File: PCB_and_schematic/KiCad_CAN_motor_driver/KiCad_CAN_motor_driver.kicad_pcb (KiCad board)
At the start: 2 copper layers, 90.4 x 45.2 mm, 75 parts, among them J1 SWDIO, J2 UART, J3 POWER IN 24V, J4 MOTOR OUT, J5 CAN, J6 PWM_IN, Q1 BTN8982TA, Q2 BTN8982TA, U1 SN65HVD232, U2 LMR50410, U3 STM32F103C8Tx

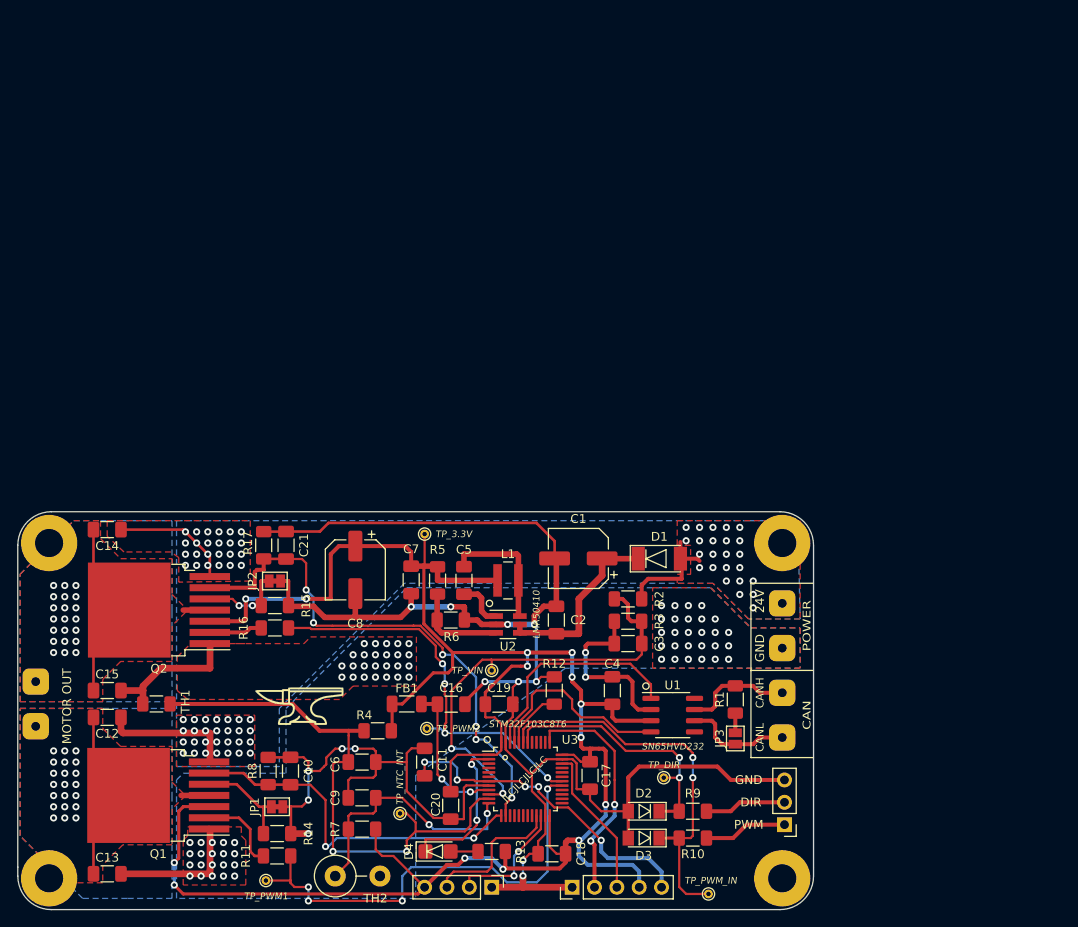
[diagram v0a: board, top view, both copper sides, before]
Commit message: PCB and schematic rev 1.1
+ revision 1.1 of schematic and PCB
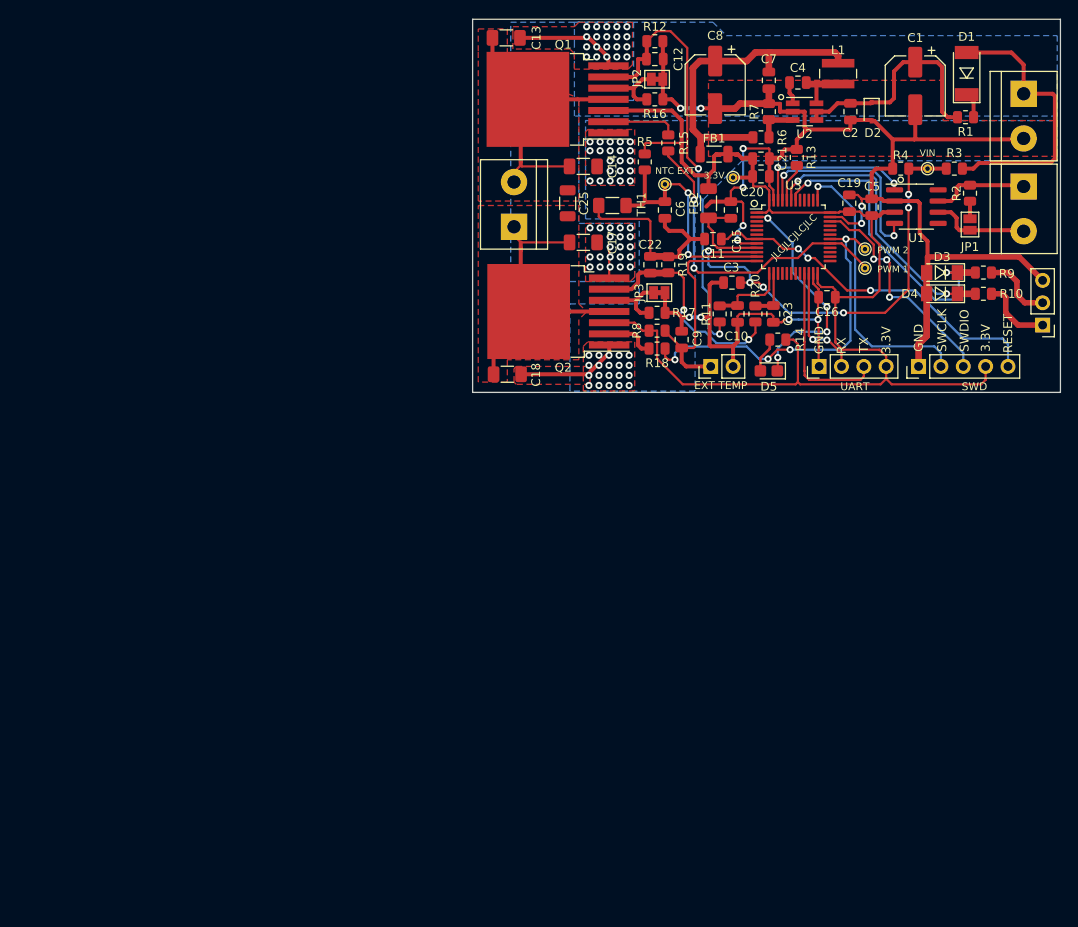
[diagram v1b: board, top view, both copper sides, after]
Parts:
- removed the G*** at (169.9, 81.0)
- removed the G*** at (137.9, 99.1)
- removed MountHole (x4): MountingHole_3.2mm_M3_Pad, MountingHole:MountingHole_3.2mm_M3_Pad
- removed REF**: OSHW-Logo2_7.3x6mm_SilkScreen, Symbol:OSHW-Logo2_7.3x6mm_SilkScreen
- removed REF**: KiCad-Logo2_5mm_SilkScreen, Symbol:KiCad-Logo2_5mm_SilkScreen
- removed TP_3.3V: 3V3, TestPoint:TestPoint_THTPad_D1.0mm_Drill0.5mm
- removed TP_DIR: DIR, TestPoint:TestPoint_THTPad_D1.0mm_Drill0.5mm
- removed TP_NTC_INT: NTC INT, TestPoint:TestPoint_THTPad_D1.0mm_Drill0.5mm
- removed TP_PWM1: PWM OUT 1, TestPoint:TestPoint_THTPad_D1.0mm_Drill0.5mm
- removed TP_PWM2: PWM OUT 2, TestPoint:TestPoint_THTPad_D1.0mm_Drill0.5mm
- removed TP_PWM_IN: PWM IN, TestPoint:TestPoint_THTPad_D1.0mm_Drill0.5mm
- removed TP_VIN: VIN, TestPoint:TestPoint_THTPad_D1.0mm_Drill0.5mm
- added C22: 10nF, Capacitor_SMD:C_0805_2012Metric, F.Cu at (177.8, 48.9)
- added C23: 10nF, Capacitor_SMD:C_0805_2012Metric, F.Cu at (191.8, 54.5)
- added C25: 100nF, Capacitor_SMD:C_1206_3216Metric, F.Cu at (168.4, 41.9)
- added D5: LED, LED_SMD:LED_0805_2012Metric_Castellated, F.Cu at (191.3, 61.0)
- added FB2: Ferrite_Bead, Inductor_SMD:L_1206_3216Metric_Pad1.22x1.90mm_HandSolder, F.Cu at (184.4, 41.9)
- added G***: LOGO, WK_lib:Anvil_10x10mm, B.Cu at (193.4, 24.1)
- added R18: 1k, Resistor_SMD:R_0805_2012Metric, F.Cu at (178.6, 58.4)
- added R19: 470R, Resistor_SMD:R_0805_2012Metric, F.Cu at (179.8, 48.9)
- added R20: 33k, Resistor_SMD:R_0805_2012Metric, F.Cu at (189.7, 54.5)
- added TP1: VIN, TestPoint:TestPoint_THTPad_D1.0mm_Drill0.5mm, F.Cu at (209.3, 38.0)
- added TP2: NTC INT, TestPoint:TestPoint_THTPad_D1.0mm_Drill0.5mm, F.Cu at (179.5, 39.8)
- added TP3: 3V3, TestPoint:TestPoint_THTPad_D1.0mm_Drill0.5mm, F.Cu at (187.2, 39.0)
- added TP5: PWM OUT 1, TestPoint:TestPoint_THTPad_D1.0mm_Drill0.5mm, F.Cu at (202.2, 49.3)
- added TP7: PWM OUT 2, TestPoint:TestPoint_THTPad_D1.0mm_Drill0.5mm, F.Cu at (202.2, 47.1)
- C10, C11, C16, C19, C2, C20, C3, C4, C5, C6, C7, C9: footprint Capacitor_SMD:C_1206_3216Metric_Pad1.33x1.80mm_HandSolder -> Capacitor_SMD:C_0805_2012Metric
- C12: value 220nF -> 10nF; footprint Capacitor_SMD:C_1206_3216Metric_Pad1.33x1.80mm_HandSolder -> Capacitor_SMD:C_0805_2012Metric
- C15: value 220nF -> 100nF; footprint Capacitor_SMD:C_1206_3216Metric_Pad1.33x1.80mm_HandSolder -> Capacitor_SMD:C_0805_2012Metric
- C17, C18: value 100nF -> 220nF
- C21: value 10nF -> 100nF; footprint Capacitor_SMD:C_1206_3216Metric_Pad1.33x1.80mm_HandSolder -> Capacitor_SMD:C_0805_2012Metric
- D2: value 3V -> SD24_SOD323; footprint Diode_SMD:D_MiniMELF -> Diode_SMD:D_SOD-323
- D4: value LED -> 3V; footprint LED_SMD:LED_1206_3216Metric_Castellated -> Diode_SMD:D_MiniMELF
- FB1: footprint Inductor_SMD:L_1206_3216Metric_Pad1.22x1.90mm_HandSolder -> Inductor_SMD:L_1206_3216Metric
- J3: value POWER IN 24V -> PWM_IN; footprint WK_lib:PowerPad_2x_3mm -> Connector_PinHeader_2.54mm:PinHeader_1x03_P2.54mm_Vertical
- J4: value MOTOR OUT -> POWER IN 24V; footprint WK_lib:PowerPad_2x_3mm -> WK_lib:ScrewTerminal_2_P5.08mm
- J5: value CAN -> MOTOR OUT; footprint WK_lib:PowerPad_2x_3mm -> WK_lib:ScrewTerminal_2_P5.08mm
- J6: value PWM_IN -> CAN; footprint Connector_PinHeader_2.54mm:PinHeader_1x03_P2.54mm_Vertical -> WK_lib:ScrewTerminal_2_P5.08mm
- JP1: footprint Jumper:SolderJumper-2_P1.3mm_Bridged_Pad1.0x1.5mm -> Jumper:SolderJumper-2_P1.3mm_Open_Pad1.0x1.5mm
- JP3: footprint Jumper:SolderJumper-2_P1.3mm_Open_Pad1.0x1.5mm -> Jumper:SolderJumper-2_P1.3mm_Bridged_Pad1.0x1.5mm
- R1: value 120R -> 10R; footprint Resistor_SMD:R_1206_3216Metric_Pad1.30x1.75mm_HandSolder -> Resistor_SMD:R_0805_2012Metric
- R10, R17, R9: footprint Resistor_SMD:R_1206_3216Metric_Pad1.30x1.75mm_HandSolder -> Resistor_SMD:R_0805_2012Metric
- R11: value 1k -> 33k; footprint Resistor_SMD:R_1206_3216Metric_Pad1.30x1.75mm_HandSolder -> Resistor_SMD:R_0805_2012Metric
- R12: value 10k -> 470R; footprint Resistor_SMD:R_1206_3216Metric_Pad1.30x1.75mm_HandSolder -> Resistor_SMD:R_0805_2012Metric
- R13: value 1.5k -> 10k; footprint Resistor_SMD:R_1206_3216Metric_Pad1.30x1.75mm_HandSolder -> Resistor_SMD:R_0805_2012Metric
- R14: value 470R -> 1.1k; footprint Resistor_SMD:R_1206_3216Metric_Pad1.30x1.75mm_HandSolder -> Resistor_SMD:R_0805_2012Metric
- R15: value 470R -> 1k; footprint Resistor_SMD:R_1206_3216Metric_Pad1.30x1.75mm_HandSolder -> Resistor_SMD:R_0805_2012Metric
- R16: value 1k -> 470R; footprint Resistor_SMD:R_1206_3216Metric_Pad1.30x1.75mm_HandSolder -> Resistor_SMD:R_0805_2012Metric
- R2: value 10k -> 120R; footprint Resistor_SMD:R_1206_3216Metric_Pad1.30x1.75mm_HandSolder -> Resistor_SMD:R_0805_2012Metric
- R3: value 1.1k -> 10k; footprint Resistor_SMD:R_1206_3216Metric_Pad1.30x1.75mm_HandSolder -> Resistor_SMD:R_0805_2012Metric
- R4: value 10k -> 1.1k; footprint Resistor_SMD:R_1206_3216Metric_Pad1.30x1.75mm_HandSolder -> Resistor_SMD:R_0805_2012Metric
- R5: value 51k -> 10k; footprint Resistor_SMD:R_1206_3216Metric_Pad1.30x1.75mm_HandSolder -> Resistor_SMD:R_0805_2012Metric
- R6: value 22k -> 51k; footprint Resistor_SMD:R_1206_3216Metric_Pad1.30x1.75mm_HandSolder -> Resistor_SMD:R_0805_2012Metric
- R7: value 10k -> 22k; footprint Resistor_SMD:R_1206_3216Metric_Pad1.30x1.75mm_HandSolder -> Resistor_SMD:R_0805_2012Metric
- R8: value 470R -> 10k; footprint Resistor_SMD:R_1206_3216Metric_Pad1.30x1.75mm_HandSolder -> Resistor_SMD:R_0805_2012Metric
- TH2: footprint Resistor_THT:R_Axial_DIN0414_L11.9mm_D4.5mm_P5.08mm_Vertical -> Connector_PinHeader_2.54mm:PinHeader_1x02_P2.54mm_Vertical
- moved J4 132.0 mm to (220.2, 29.5)
- moved C13 105.3 mm to (161.4, 23.1), turned to 180 degrees
- moved JP1 102.8 mm to (214.1, 44.3), turned to 270 degrees
- moved C12 97.3 mm to (178.3, 25.5), turned to 0 degrees
- moved R7 93.7 mm to (191.3, 31.5), turned to 90 degrees
- moved Q1 91.2 mm to (167.3, 30.1)
- moved C15 89.5 mm to (186.9, 42.7), turned to 90 degrees
- moved R4 87.3 mm to (206.2, 38.0)
- moved R13 86.2 mm to (194.4, 36.7), turned to 270 degrees
- moved D4 85.4 mm to (210.9, 52.2), turned to 180 degrees
- moved D2 83.6 mm to (202.9, 31.5), turned to 270 degrees
- moved R14 79.9 mm to (192.3, 57.4), turned to 180 degrees
- moved C20 79.7 mm to (190.4, 38.9), turned to 0 degrees
- moved R11 79.5 mm to (185.7, 54.5), turned to 270 degrees
- moved J6 77.4 mm to (220.2, 40.0), turned to 270 degrees
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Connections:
- C12 pad 1: +24V -> Net-(C12-Pad1)
- C12 pad 2: /MOT_A -> GND
- C13 pad 1: /MOT_A -> +24V
- C13 pad 2: GND -> /MOT_A
- C14 pad 1: +24V -> /MOT_A
- C14 pad 2: /MOT_B -> GND
- C15 pad 1: /MOT_B -> Net-(C15-Pad1)
- C16 pad 1: Net-(C16-Pad1) -> +3V3
- C17 pad 1: +3V3 -> +24V
- C17 pad 2: GND -> /MOT_B
- C18 pad 1: +3V3 -> /MOT_B
- C21 pad 1: /I_SENSE_2 -> +3V3
- C4 pad 1: +3V3 -> Net-(C4-Pad1)
- C4 pad 2: GND -> Net-(C4-Pad2)
- C5 pad 1: Net-(C5-Pad1) -> +3V3
- C5 pad 2: Net-(C5-Pad2) -> GND
- C7 pad 1: +3V3 -> Net-(C7-Pad1)
- C8 pad 1: +3V3 -> Net-(C7-Pad1)
- D1 pad 1: Net-(C1-Pad1) -> Net-(D1-Pad1)
- D2 pad 1: Net-(D2-Pad1) -> Net-(C1-Pad1)
- D4 pad 2: Net-(D4-Pad2) -> GND
- FB1 pad 2: Net-(C16-Pad1) -> Net-(C7-Pad1)
- J3 pad 1: GND -> /PWM_IN
- J3 pad 2: +24V -> /DIR_IN
- J4 pad 1: /MOT_B -> +24V
- J4 pad 2: /MOT_A -> GND
- J5 pad 1: /CAN_L -> /MOT_B
- J5 pad 2: /CAN_H -> /MOT_A
- J6 pad 1: /PWM_IN -> /CAN_H
- J6 pad 2: /DIR_IN -> /CAN_L
- JP1 pad 2: GND -> /CAN_L
- JP3 pad 2: /CAN_L -> GND
- L1 pad 1: Net-(C5-Pad2) -> Net-(C4-Pad2)
- L1 pad 2: +3V3 -> Net-(C7-Pad1)
- Q1 pad 5: Net-(JP1-Pad1) -> Net-(JP2-Pad1)
- Q1 pad 6: /I_SENSE_1 -> Net-(C12-Pad1)
- Q2 pad 5: Net-(JP2-Pad1) -> Net-(JP3-Pad1)
- Q2 pad 6: /I_SENSE_2 -> Net-(C22-Pad1)
- R1 pad 1: /CAN_H -> Net-(D1-Pad1)
- R1 pad 2: Net-(JP3-Pad1) -> Net-(C1-Pad1)
- R10 pad 2: Net-(D3-Pad1) -> Net-(D4-Pad1)
- R11 pad 1: /PWM_1 -> /I_SENSE_1
- R11 pad 2: Net-(Q1-Pad2) -> Net-(C12-Pad1)
- R12 pad 1: GND -> Net-(C12-Pad1)
- R12 pad 2: Net-(R12-Pad2) -> GND
- R13 pad 1: +3V3 -> GND
- R13 pad 2: Net-(D4-Pad2) -> Net-(R13-Pad2)
- R14 pad 1: Net-(JP1-Pad1) -> +3V3
- R14 pad 2: GND -> Net-(D5-Pad2)
- R15 pad 1: Net-(JP2-Pad1) -> /PWM_1
- R15 pad 2: GND -> Net-(Q1-Pad2)
- R16 pad 1: Net-(Q2-Pad2) -> Net-(JP2-Pad1)
- R16 pad 2: /PWM_2 -> GND
- R17 pad 1: /I_SENSE_2 -> Net-(JP3-Pad1)
- R2 pad 1: +24V -> /CAN_H
- R2 pad 2: /VIN -> Net-(JP1-Pad1)
- R3 pad 1: /VIN -> +24V
- R3 pad 2: GND -> /VIN
- R4 pad 1: +3V3 -> /VIN
- R4 pad 2: /NTC_INTERNAL -> GND
- R5 pad 2: Net-(R5-Pad2) -> /NTC_INTERNAL
- R6 pad 1: Net-(R5-Pad2) -> Net-(C7-Pad1)
- R6 pad 2: GND -> Net-(R6-Pad2)
- R7 pad 1: +3V3 -> Net-(R6-Pad2)
- R7 pad 2: /NTC_EXTERNAL -> GND
- R8 pad 1: /I_SENSE_1 -> +3V3
- R8 pad 2: GND -> /NTC_EXTERNAL
- R9 pad 2: Net-(D2-Pad1) -> Net-(D3-Pad1)
- U1 pad 5: Net-(U1-Pad5) -> (no net)
- U1 pad 8: Net-(U1-Pad8) -> (no net)
- U2 pad 1: Net-(C5-Pad1) -> Net-(C4-Pad1)
- U2 pad 3: Net-(R5-Pad2) -> Net-(R6-Pad2)
- U2 pad 6: Net-(C5-Pad2) -> Net-(C4-Pad2)
- U3 pad 15: Net-(U3-Pad15) -> (no net)
- U3 pad 16: Net-(U3-Pad16) -> (no net)
- U3 pad 17: Net-(U3-Pad17) -> (no net)
- U3 pad 18: Net-(U3-Pad18) -> (no net)
- U3 pad 19: Net-(U3-Pad19) -> (no net)
- U3 pad 2: Net-(D4-Pad1) -> Net-(D5-Pad1)
- U3 pad 20: Net-(U3-Pad20) -> (no net)
- U3 pad 25: Net-(U3-Pad25) -> (no net)
- U3 pad 26: Net-(U3-Pad26) -> (no net)
- U3 pad 27: Net-(U3-Pad27) -> (no net)
- U3 pad 28: Net-(U3-Pad28) -> (no net)
- U3 pad 3: Net-(U3-Pad3) -> (no net)
- U3 pad 31: Net-(U3-Pad31) -> (no net)
- U3 pad 32: Net-(U3-Pad32) -> (no net)
- U3 pad 33: Net-(U3-Pad33) -> (no net)
- U3 pad 38: Net-(U3-Pad38) -> (no net)
- U3 pad 39: Net-(U3-Pad39) -> (no net)
- U3 pad 4: Net-(U3-Pad4) -> (no net)
- U3 pad 40: Net-(U3-Pad40) -> (no net)
- U3 pad 41: Net-(U3-Pad41) -> (no net)
- U3 pad 42: Net-(D2-Pad1) -> Net-(D3-Pad1)
- U3 pad 43: Net-(D3-Pad1) -> Net-(D4-Pad1)
- U3 pad 44: Net-(R12-Pad2) -> Net-(R13-Pad2)
- U3 pad 5: Net-(U3-Pad5) -> (no net)
- U3 pad 6: Net-(U3-Pad6) -> (no net)
- U3 pad 9: Net-(C16-Pad1) -> Net-(C15-Pad1)
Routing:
- net +3V3: track 244.2 -> 145.8 mm, vias 14 -> 0
- net GND: track 292.1 -> 233.1 mm, vias 88 -> 53
- net /I_SENSE_2: track 61.2 -> 5.71 mm, vias 6 -> 0
- net Net-(C12-Pad1): track 0.00 -> 49.8 mm, vias 0 -> 2
- net Net-(C7-Pad1): track 0.00 -> 36.6 mm
- net /NTC_INTERNAL: track 64.0 -> 28.2 mm
- net /I_SENSE_1: track 41.2 -> 8.90 mm, vias 2 -> 0
- net Net-(D2-Pad1): track 30.4 -> 0.00 mm, vias 2 -> 0
- net Net-(C22-Pad1): track 0.00 -> 26.2 mm, vias 0 -> 2
- net Net-(D5-Pad1): track 0.00 -> 25.9 mm, vias 0 -> 4
- net Net-(C16-Pad1): track 16.8 -> 0.00 mm, vias 2 -> 0
- net /PWM_1: track 52.5 -> 36.8 mm, vias 4 -> 2
- net Net-(C5-Pad2): track 14.6 -> 0.00 mm
- net Net-(D4-Pad1): track 17.5 -> 32.1 mm
- net Net-(C15-Pad1): track 0.00 -> 10.9 mm
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- removed copper zone on B.Cu, net /MOT_A
- removed copper zone on B.Cu, net /MOT_B
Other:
- board size 90.4 x 45.2 mm -> 66.8 x 42.4 mm
- board text added: "CAN H"
- board text added: "CAN L"
- board text added: "EXT TEMP"
- board text added: "NTC EXT"
- board text added: "PWM 1"
- board text added: "PWM 2"
- board text added: "RST"
- board text added: "RX"
- board text added: "Rev 1.1"
- board text added: "TX"
- board text added: "VIN"
- board text removed: "24V"
- board text removed: "CAN"
- board text removed: "CAN HIGH"
- board text removed: "CAN LOW"
- board text removed: "CANH"
- board text removed: "CANL"
- board text removed: "LMR50410"
- board text removed: "POWER"
- board text removed: "Rev 1.0"
- board text removed: "SN65HVD232"
- board text removed: "STM32F103C8T6"
